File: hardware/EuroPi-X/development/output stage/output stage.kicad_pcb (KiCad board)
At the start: 2 copper layers, 20.3 x 15.2 mm, 27 parts, among them J1 Conn_01x06_Pin, J2 Conn_01x06_Pin, U1 TL074

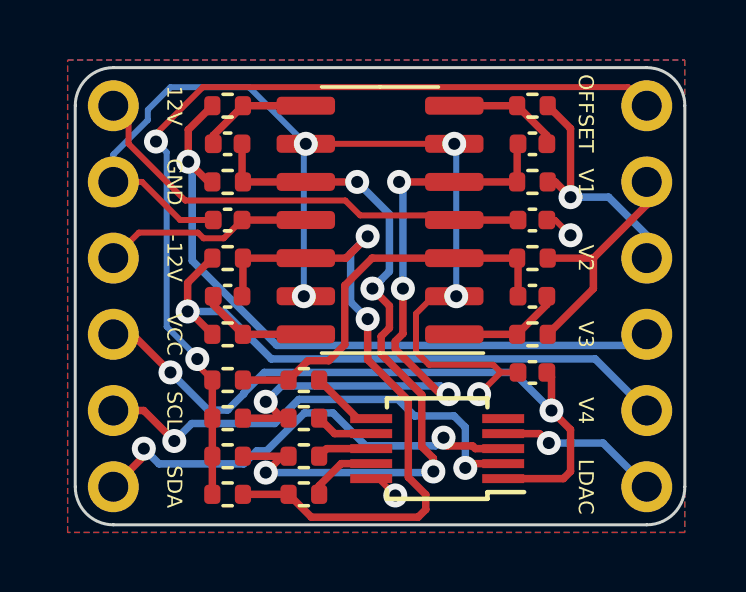
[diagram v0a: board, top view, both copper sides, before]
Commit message: save
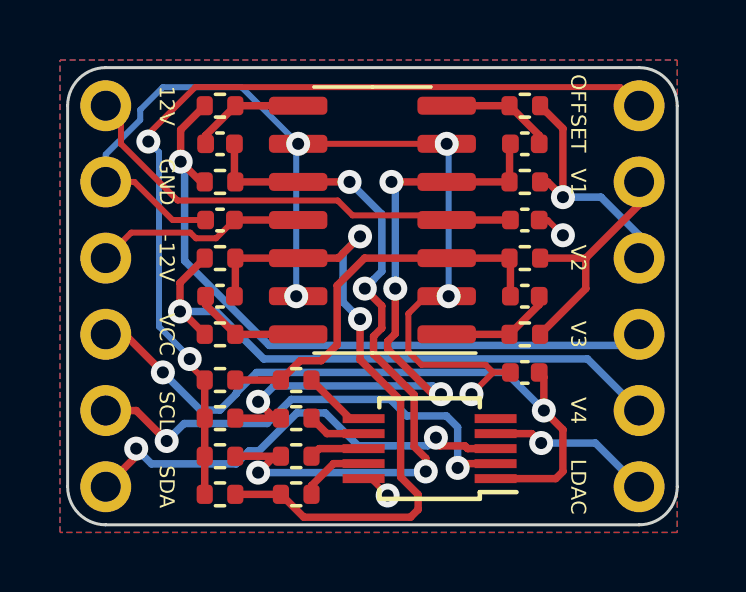
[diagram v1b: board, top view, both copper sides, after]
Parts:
- moved DAC1 0.25 mm to (12.1, 12.7)
- moved J1 0.25 mm to (1.27, 1.27)
- moved C1 0.25 mm to (15.2, 10.2)
- moved C2 0.25 mm to (15.2, 7.62)
- moved C3 0.25 mm to (15.2, 2.54)
- moved C4 0.25 mm to (5.08, 2.54)
- moved C5 0.25 mm to (5.08, 7.62)
- moved C6 0.25 mm to (15.2, 5.08)
- moved C7 0.25 mm to (5.08, 5.08)
- moved R1 0.25 mm to (5.08, 10.4)
- moved R10 0.25 mm to (7.62, 13.0)
- moved R11 0.25 mm to (5.08, 3.81)
- moved R12 0.25 mm to (5.08, 1.27)
- moved R13 0.25 mm to (5.08, 14.2)
- moved R14 0.25 mm to (7.62, 14.2)
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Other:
- outline, holes or cut-outs redrawn
